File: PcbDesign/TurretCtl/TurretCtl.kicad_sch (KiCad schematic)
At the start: 17 parts, among them J1 FLIR, J2 Stepper1, J3 Stepper2, J4 PWR, J5 Sensors

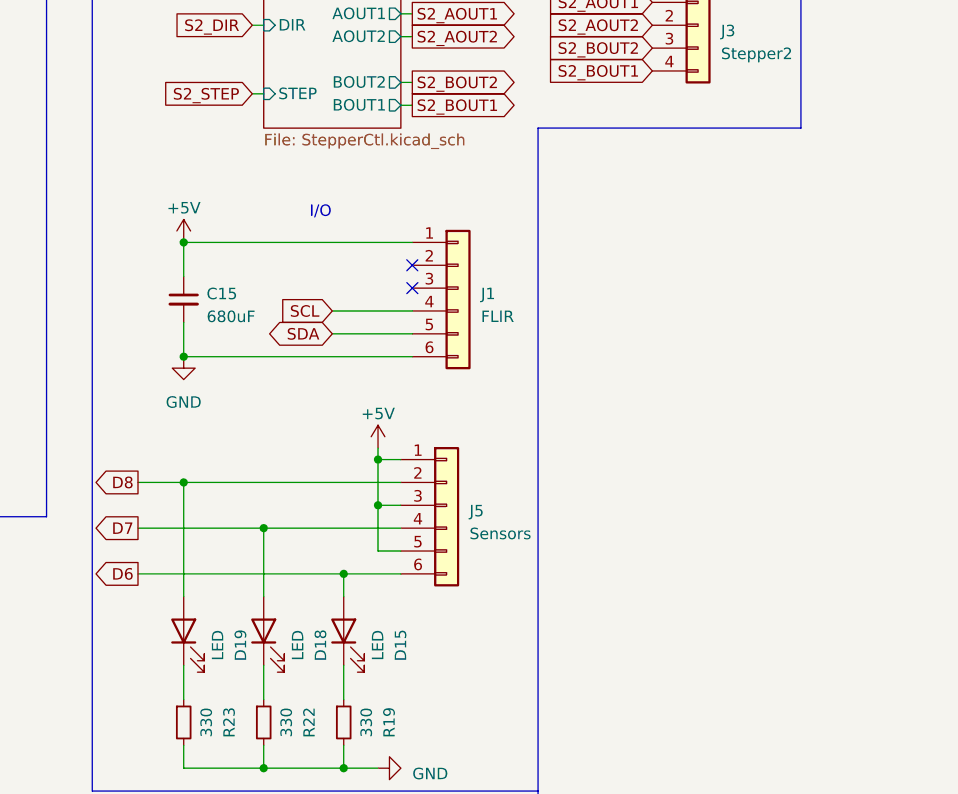
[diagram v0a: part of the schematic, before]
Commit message: New connectors
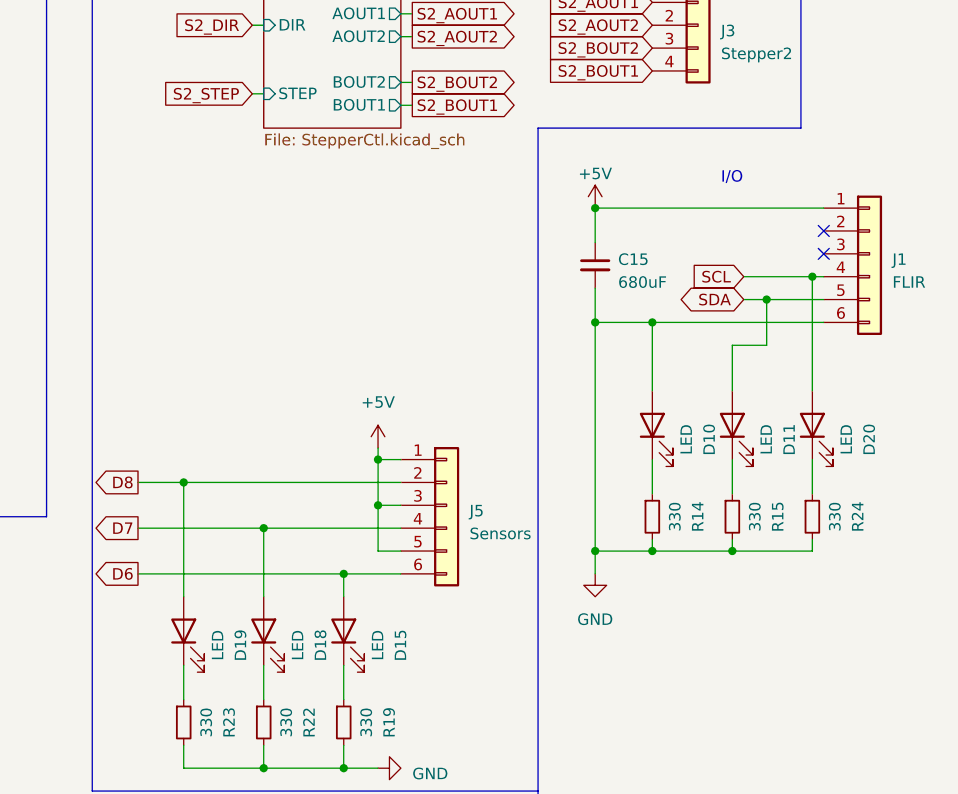
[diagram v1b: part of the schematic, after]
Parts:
- added D10, D11, D20: LED, LED_SMD:LED_0603_1608Metric, symbol Device:LED
- added R14, R15, R24: 330, Resistor_SMD:R_0402_1005Metric, symbol Device:R_Small
- J1, J5: footprint Connector_JST:JST_GH_SM06B-GHS-TB_1x06-1MP_P1.25mm_Horizontal -> Connector_Phoenix_MC:PhoenixContact_MCV_1,5_6-G-3.5_1x06_P3.50mm_Vertical
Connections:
- net GND: now also D10.2 (A), R14.2, R15.2, R24.2
- net SCL: now also D20.2 (A)
- net SDA: now also D11.2 (A)
- new net: D11.1 (K), R15.1
- new net: D20.1 (K), R24.1
- new net: D10.1 (K), R14.1
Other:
- moved on the sheet: C15, J1

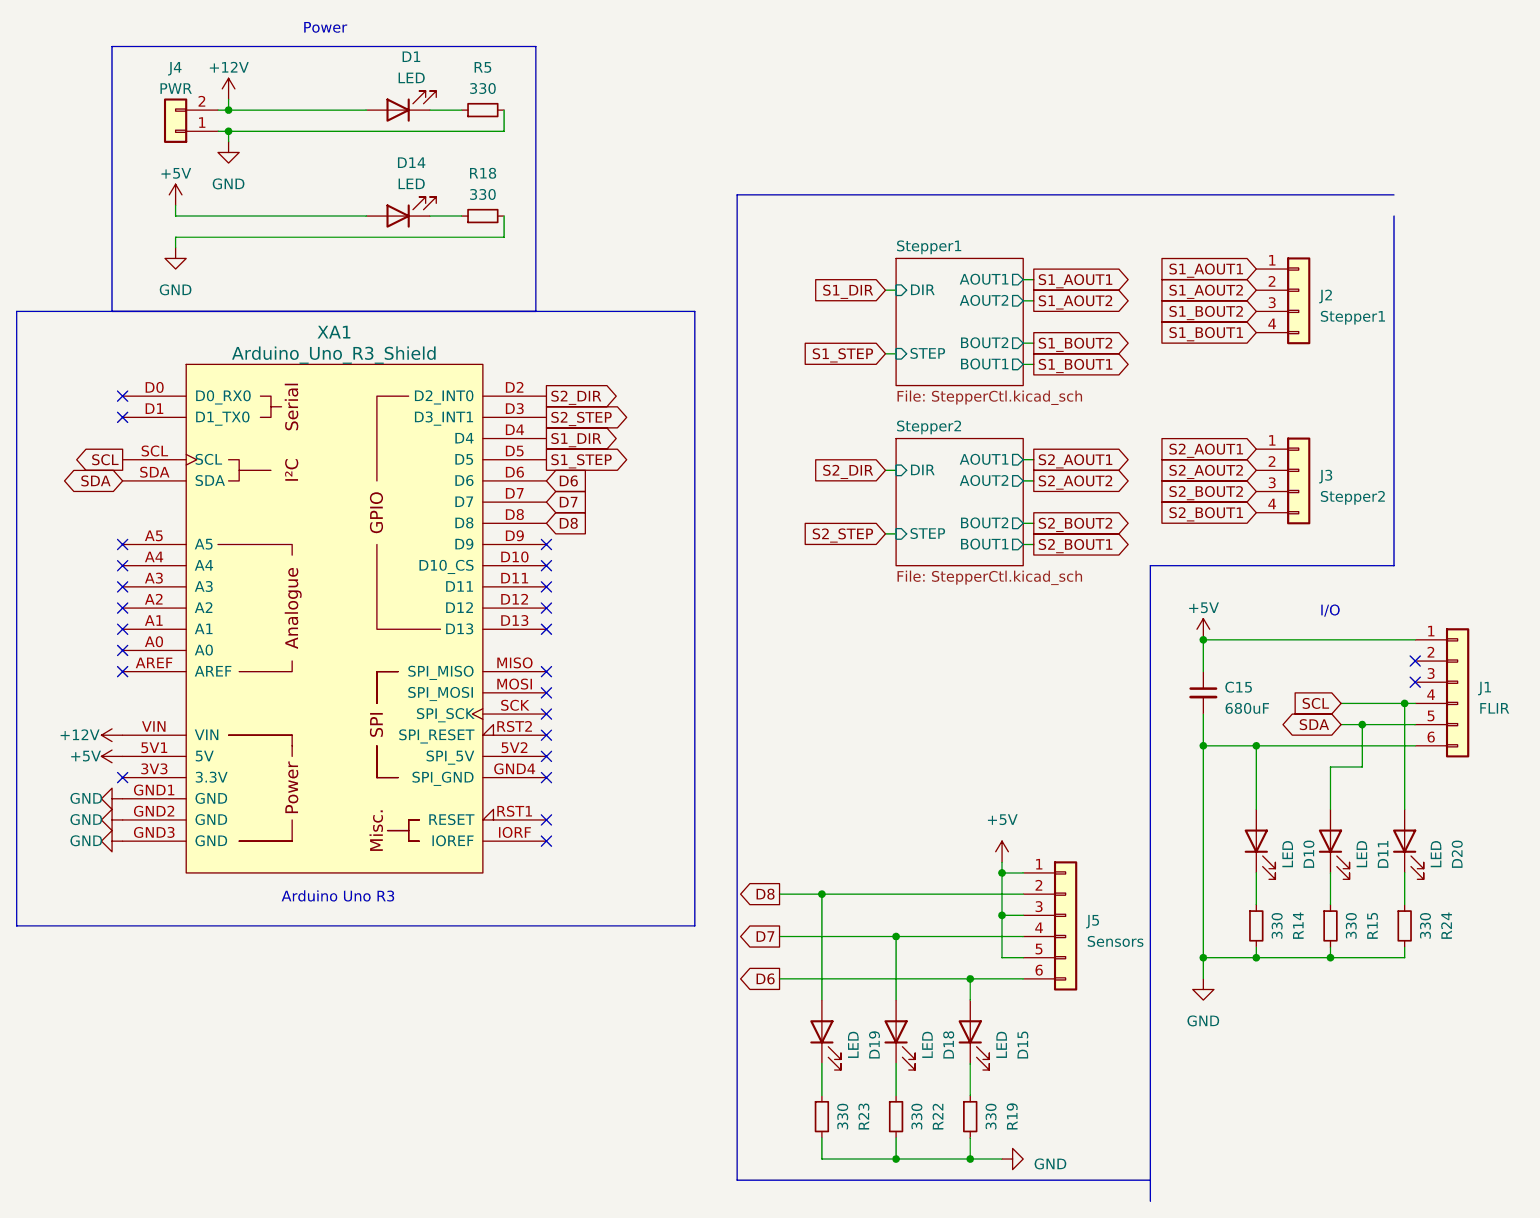
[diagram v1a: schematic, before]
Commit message: Control board v3
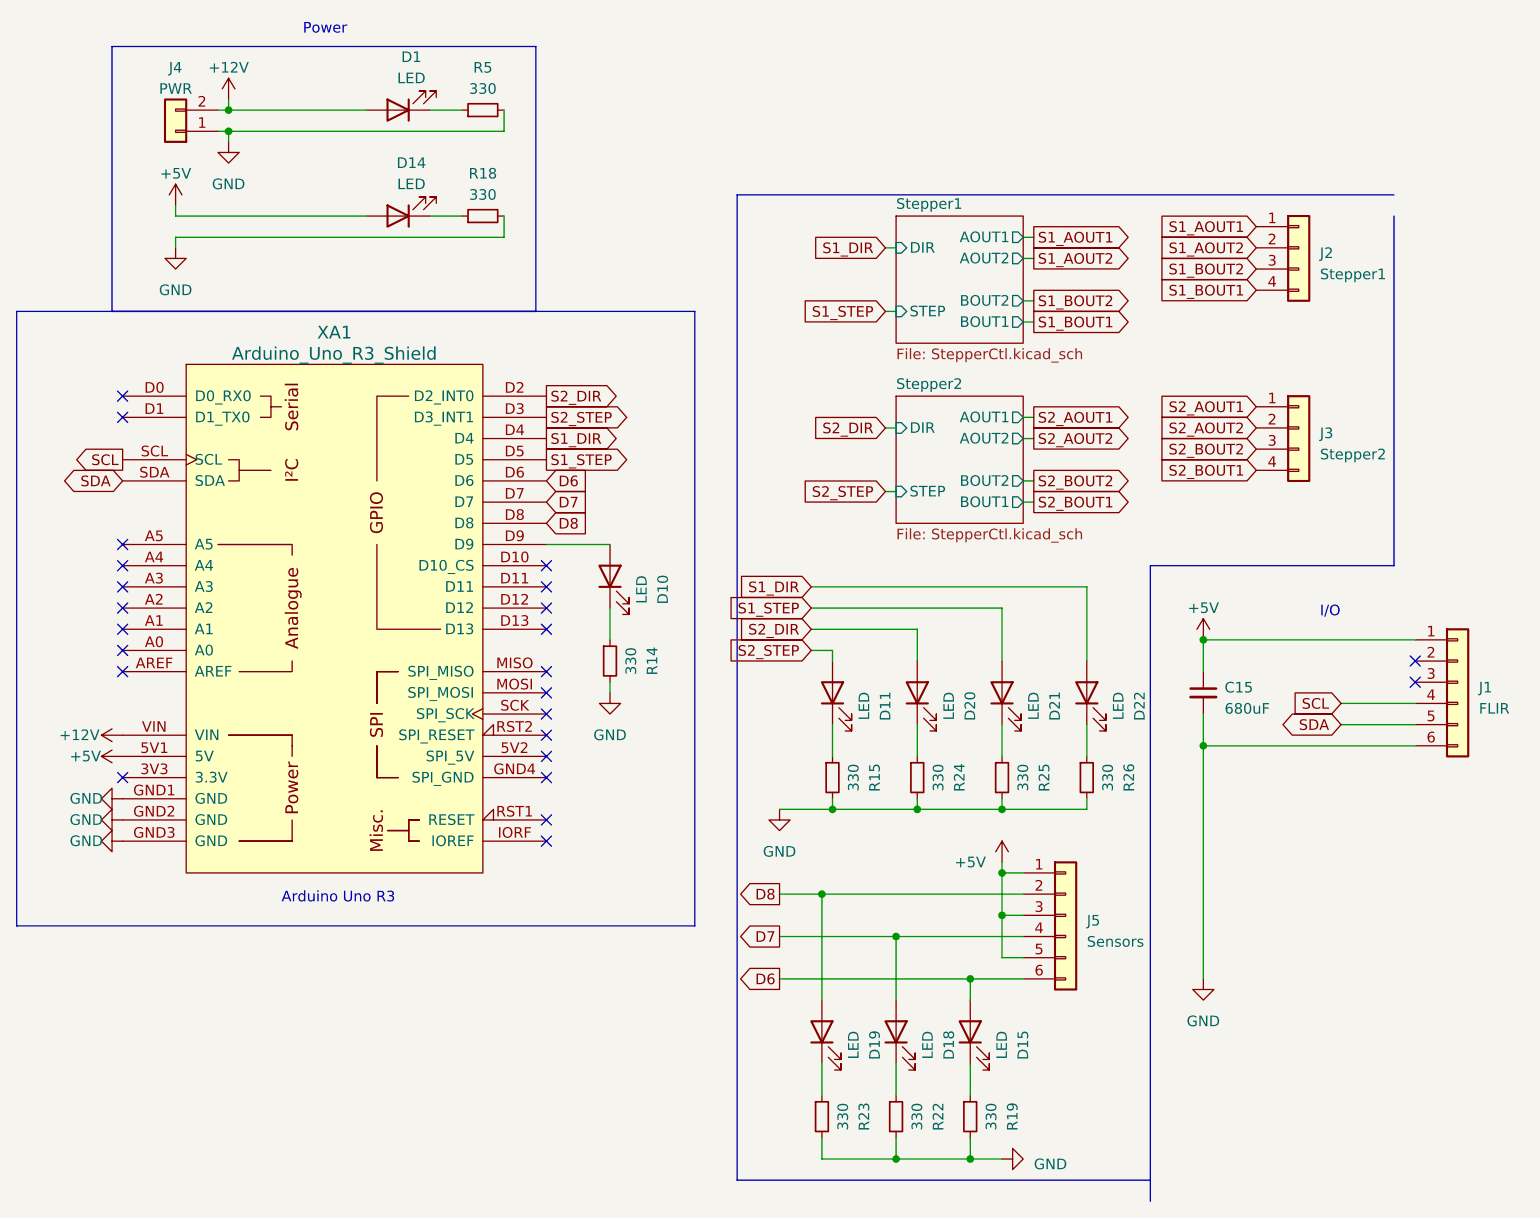
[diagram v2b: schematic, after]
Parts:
- added D21, D22: LED, LED_SMD:LED_0603_1608Metric, symbol Device:LED
- added R25, R26: 330, Resistor_SMD:R_0402_1005Metric, symbol Device:R_Small
- J1, J5: LCSC Part C133065 -> (none); LCSC Part # C133065 -> (none)
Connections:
- net GND: now also R25.2, R26.2; no longer D10.2 (A)
- net S1_DIR: now also D22.2 (A)
- net S1_STEP: now also D21.2 (A)
- net S2_DIR: now also D20.2 (A)
- net S2_STEP: now also D11.2 (A)
- net SCL: no longer D20.2 (A)
- net SDA: no longer D11.2 (A)
- net at XA1.D9: now also D10.2 (A)
- new net: D22.1 (K), R26.1
- new net: D21.1 (K), R25.1
- no-connect marks 25 -> 24
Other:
- moved on the sheet: D10, J2, J3, R14
